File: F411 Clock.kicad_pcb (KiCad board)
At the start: 2 copper layers, 4 parts, among them J1 USB_C_Receptacle_USB2.0_16P, U1 STM32F411CCUx

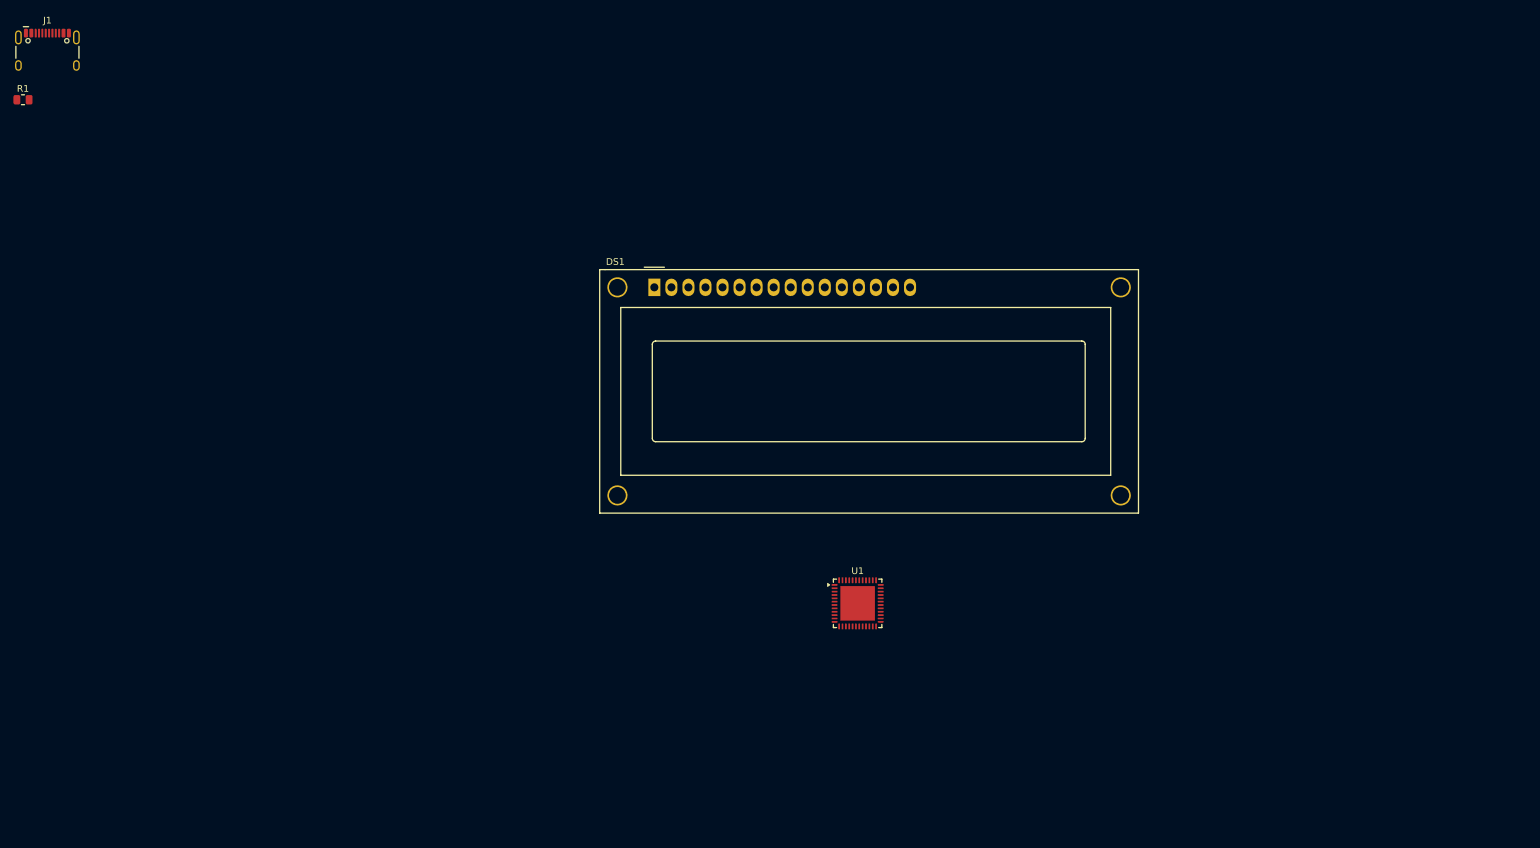
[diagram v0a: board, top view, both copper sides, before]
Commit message: Close: 3 files changed F411 Clock.kicad_pcb 0/0/3 F411 Clock.kicad_prl 138/0/0 F411 Clock.kicad_pro 651/0/0
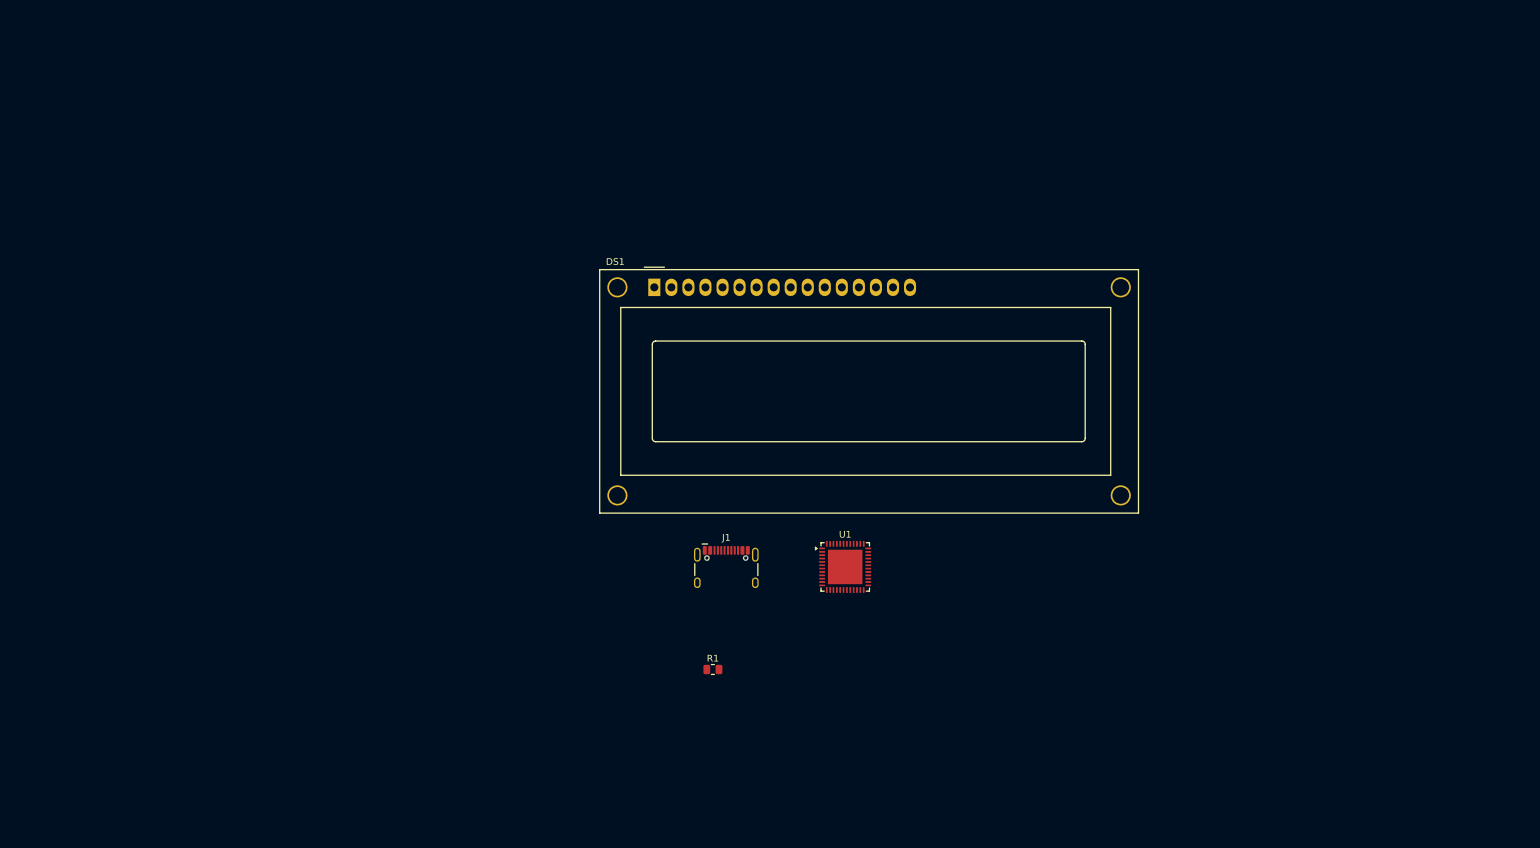
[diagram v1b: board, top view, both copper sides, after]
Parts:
- moved R1 133.3 mm to (104.5, 96.0)
- moved J1 127.2 mm to (106.5, 82.0)
- moved U1 5.73 mm to (124.2, 80.7)
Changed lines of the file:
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@@
 	(footprint "Connector_USB:USB_C_Receptacle_HCTL_HC-TYPE-C-16P-01A"
 		(layer "F.Cu")
-		(at 5.345 4.925)
+		(at 106.5 82)
 		(descr "16-pin USB-C receptacle, USB2.0 and PD, 5A VBUS rating, https://datasheet.lcsc.com/lcsc/2211161000_HCTL-HC-TYPE-C-16P-01A_C2894897.pdf")
 		(tags "usb usb-c 2.0 pd")
@@
 	(footprint "Resistor_SMD:R_0805_2012Metric"
 		(layer "F.Cu")
-		(at 1.705 11.105)
+		(at 104.5 96)
 		(descr "Resistor SMD 0805 (2012 Metric), square (rectangular) end terminal, IPC-7351 nominal, (Body size source: IPC-SM-782 page 72, https://www.pcb-3d.com/wordpress/wp-content/uploads/ipc-sm-782a_amendment_1_and_2.pdf)")
 		(tags "resistor")
@@
 	(footprint "Package_DFN_QFN:QFN-48-1EP_7x7mm_P0.5mm_EP5.15x5.15mm"
 		(layer "F.Cu")
-		(at 126.065 86.145)
+		(at 124.22 80.72)
 		(descr "QFN, 48 Pin (http://www.analog.com/media/en/package-pcb-resources/package/pkg_pdf/ltc-legacy-qfn/QFN_48_05-08-1704.pdf)")
 		(tags "QFN NoLead")

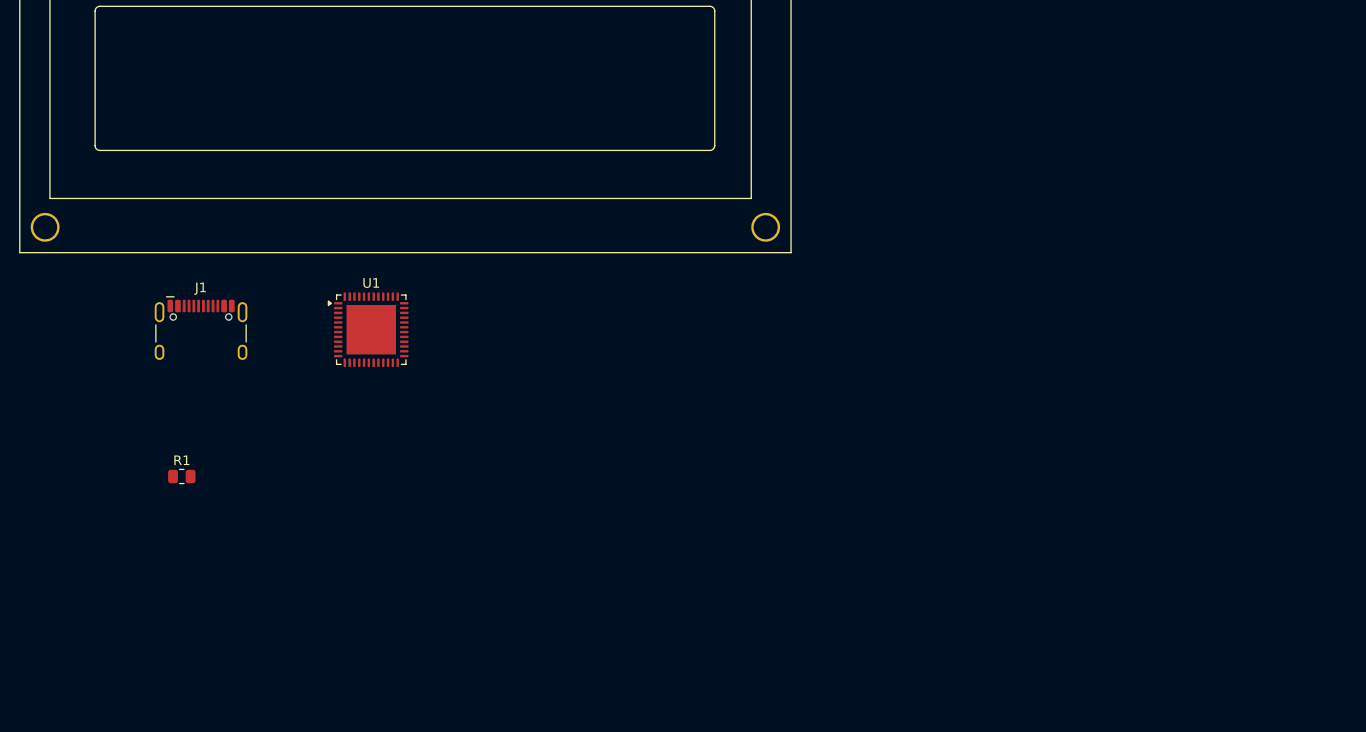
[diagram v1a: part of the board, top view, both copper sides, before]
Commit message: PCB Save: 2 files changed F411 Clock.kicad_pcb 6362/0/1538 ~F411 Clock.kicad_pcb.lck 1/0/0
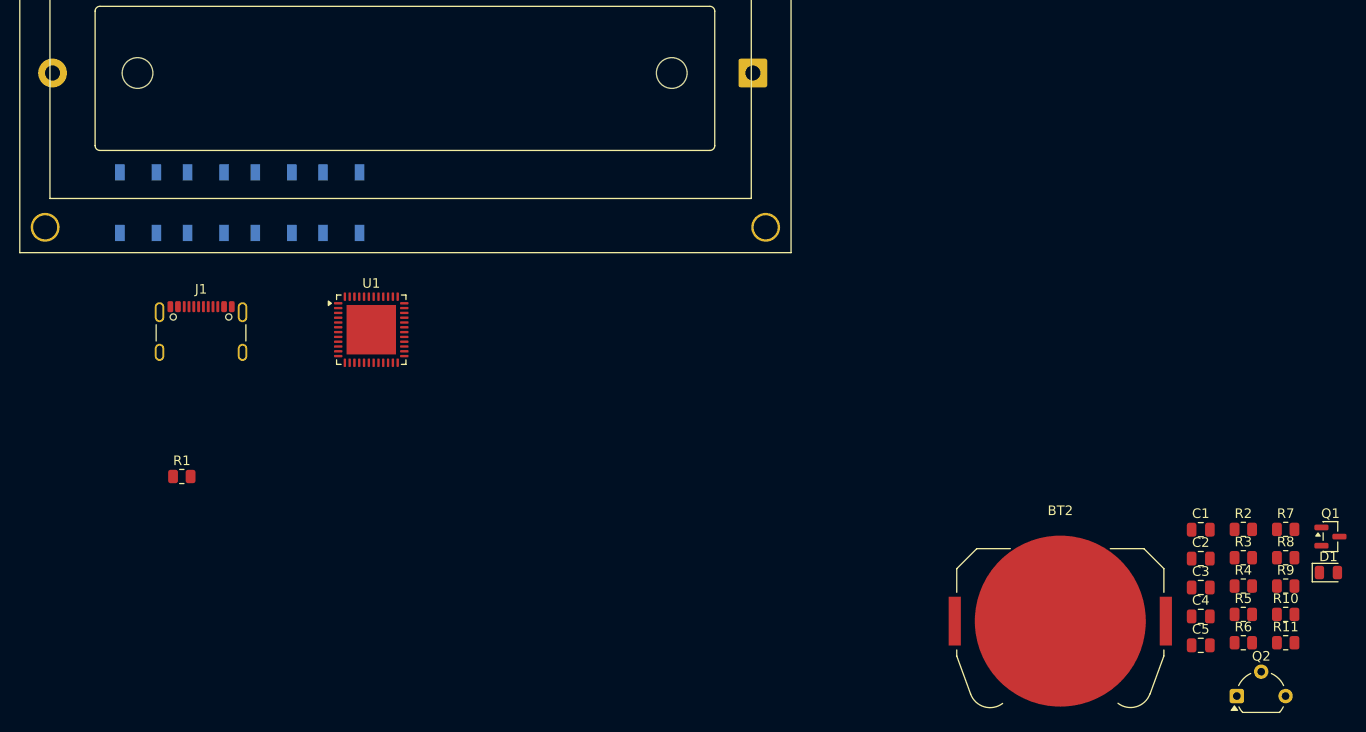
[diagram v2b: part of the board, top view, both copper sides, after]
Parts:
- added BT1: Battery, Battery:BatteryHolder_MPD_BK-18650-PC2, B.Cu at (163.9, 54.0)
- added BT2: Battery_Cell, Battery:BatteryHolder_Keystone_3034_1x20mm, F.Cu at (195.9, 111.1)
- added C1: 10uf, Capacitor_SMD:C_0805_2012Metric, F.Cu at (210.6, 101.5)
- added C2: 10uf, Capacitor_SMD:C_0805_2012Metric, F.Cu at (210.6, 104.5)
- added C3: 10uf, Capacitor_SMD:C_0805_2012Metric, F.Cu at (210.6, 107.6)
- added C4: 10uf, Capacitor_SMD:C_0805_2012Metric, F.Cu at (210.6, 110.6)
- added C5: 10uf, Capacitor_SMD:C_0805_2012Metric, F.Cu at (210.6, 113.6)
- added D1: 1N5819, Diode_SMD:D_0805_2012Metric, F.Cu at (223.9, 106.0)
- added Q1: DMG3415U, Package_TO_SOT_SMD:SOT-23, F.Cu at (224.1, 102.3)
- added Q2: BC547, Package_TO_SOT_THT:TO-92L_Wide, F.Cu at (214.3, 118.9)
- added R10: 10k, Resistor_SMD:R_0805_2012Metric, F.Cu at (219.4, 110.4)
- added R11: 10k, Resistor_SMD:R_0805_2012Metric, F.Cu at (219.4, 113.3)
- added R2: 10k, Resistor_SMD:R_0805_2012Metric, F.Cu at (215.0, 101.5)
- added R3: 5.2k, Resistor_SMD:R_0805_2012Metric, F.Cu at (215.0, 104.5)
- added R4: 5.2k, Resistor_SMD:R_0805_2012Metric, F.Cu at (215.0, 107.4)
- added R5: 10k, Resistor_SMD:R_0805_2012Metric, F.Cu at (215.0, 110.4)
- added R6: 10k, Resistor_SMD:R_0805_2012Metric, F.Cu at (215.0, 113.3)
- added R7: 10k, Resistor_SMD:R_0805_2012Metric, F.Cu at (219.4, 101.5)
- added R8: 10k, Resistor_SMD:R_0805_2012Metric, F.Cu at (219.4, 104.5)
- added R9: 10k, Resistor_SMD:R_0805_2012Metric, F.Cu at (219.4, 107.4)
- added SW1: SW_Push, Button_Switch_SMD:SW_SPST_TL3342, B.Cu at (121.1, 67.5)
- added SW2: SW_Push, Button_Switch_SMD:SW_SPST_TL3342, B.Cu at (114.0, 67.5)
- added SW3: SW_Push, Button_Switch_SMD:SW_SPST_TL3342, B.Cu at (107.0, 67.5)
- added SW4: SW_Push, Button_Switch_SMD:SW_SPST_TL3342, B.Cu at (100.0, 67.5)
- J1: footprint Connector_USB:USB_C_Receptacle_HCTL_HC-TYPE-C-16P-01A -> Connector_USB:USB_C_Receptacle_GCT_USB4105-xx-A_16P_TopMnt_Horizontal
- R1: value R_Small -> 10k
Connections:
- DS1 pad 1: unconnected-(DS1-VSS-Pad1) -> GND
- DS1 pad 15: unconnected-(DS1-LED(+)-Pad15) -> +3.3V
- DS1 pad 16: unconnected-(DS1-LED(-)-Pad16) -> Net-(DS1-LED(-))
- DS1 pad 2: unconnected-(DS1-VDD-Pad2) -> VBUS
- J1 pad A1: Net-(J1-GND-PadA1) -> GND
- J1 pad A12: Net-(J1-GND-PadA1) -> GND
- J1 pad A5: unconnected-(J1-CC1-PadA5) -> Net-(J1-CC1)
- J1 pad B1: Net-(J1-GND-PadA1) -> GND
- J1 pad B12: Net-(J1-GND-PadA1) -> GND
- J1 pad B5: unconnected-(J1-CC2-PadB5) -> Net-(J1-CC2)
- J1 pad SH: unconnected-(J1-SHIELD-PadSH) -> GND
- R1 pad 1: unconnected-(R1-Pad1) -> /DN
- R1 pad 2: unconnected-(R1-Pad2) -> Net-(J1-D--PadA7)
- U1 pad 1: unconnected-(U1-VBAT-Pad1) -> +BATT_2
- U1 pad 23: Net-(U1-VSS-Pad23) -> GND
- U1 pad 24: unconnected-(U1-VDD-Pad24) -> +3.3V
- U1 pad 32: unconnected-(U1-PA11-Pad32) -> /DN
- U1 pad 33: unconnected-(U1-PA12-Pad33) -> /DP
- U1 pad 35: Net-(U1-VSS-Pad23) -> GND
- U1 pad 36: unconnected-(U1-VDD-Pad36) -> +3.3V
- U1 pad 44: unconnected-(U1-BOOT0-Pad44) -> Net-(U1-BOOT0)
- U1 pad 47: Net-(U1-VSS-Pad23) -> GND
- U1 pad 48: unconnected-(U1-VDD-Pad48) -> +3.3V
- U1 pad 49: Net-(U1-VSS-Pad23) -> GND
- U1 pad 7: unconnected-(U1-NRST-Pad7) -> Net-(U1-NRST)
- U1 pad 8: unconnected-(U1-VSSA-Pad8) -> GND
- U1 pad 9: unconnected-(U1-VDDA-Pad9) -> +3.3AV
